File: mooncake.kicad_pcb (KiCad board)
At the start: 2 copper layers, 46 x 48.4 mm, 25 parts, among them U1 MCP23017, X1 Badgelife_shitty_connector

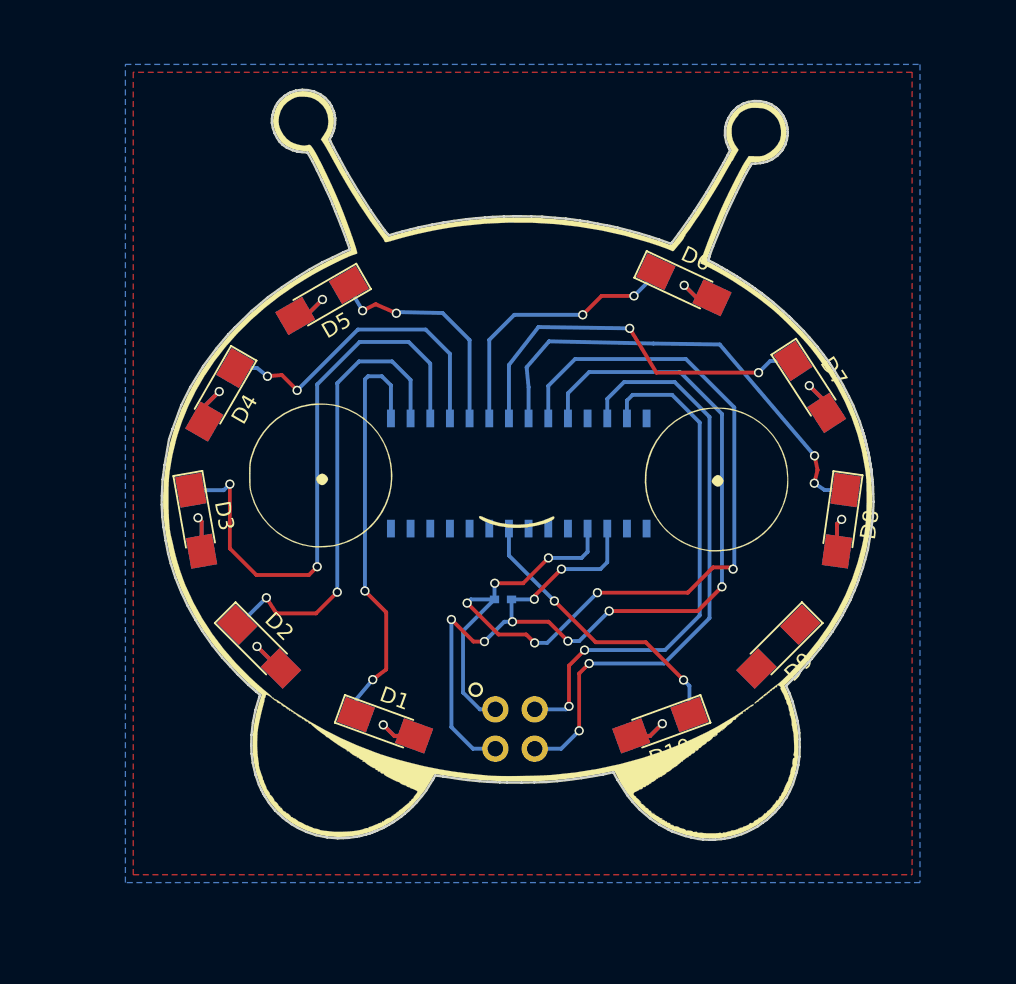
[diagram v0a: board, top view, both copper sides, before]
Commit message: Issues with EdgeCuts
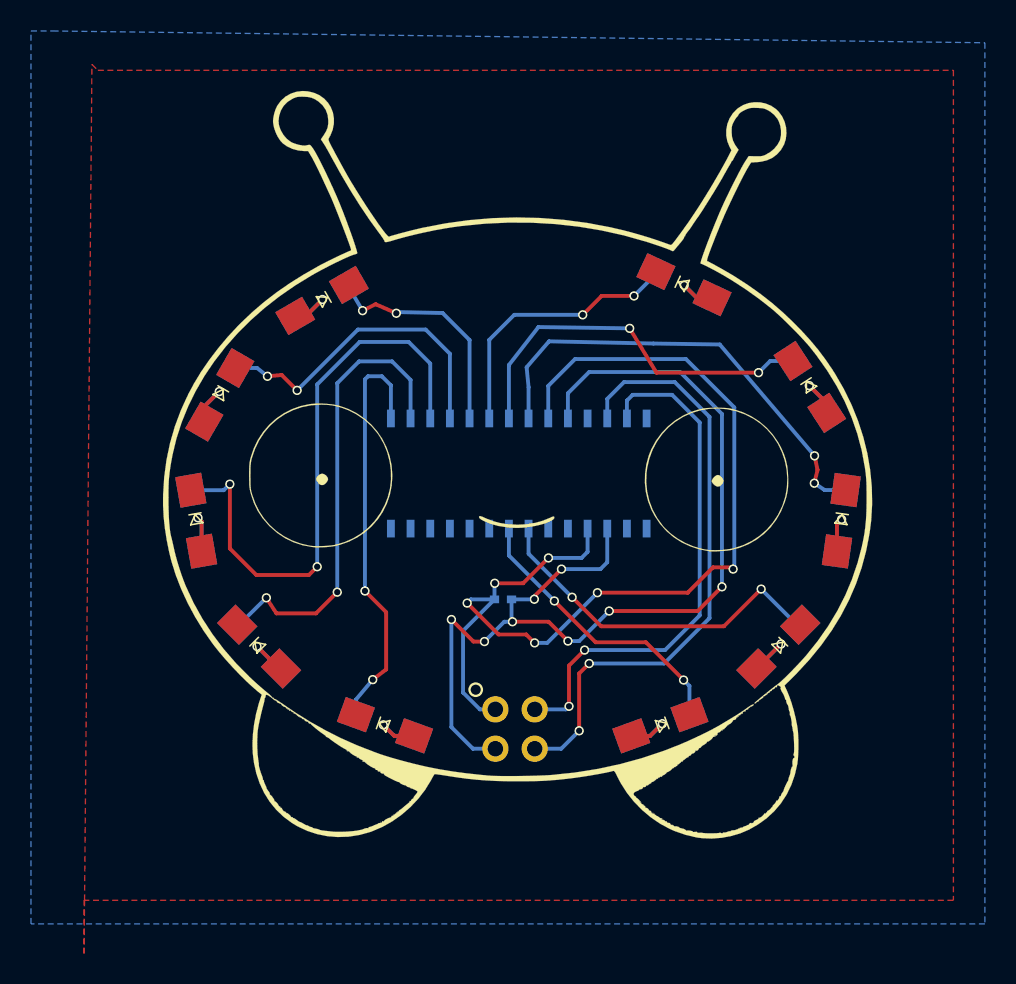
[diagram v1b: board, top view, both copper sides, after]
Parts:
- D1, D10, D2, D3, D4, D5, D6, D7, D8, D9: footprint LEDs:LED_1206_HandSoldering -> mrmeeseeks-addon-lib:LED_1206_HandSoldering_MinSilk
- R1, R10, R2, R3, R4, R5, R6, R7, R8, R9: footprint Resistors_SMD:R_1206_HandSoldering -> mrmeeseeks-addon-lib:R_1206_HandSoldering_NoSilk
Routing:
- net Net-(R9-Pad1): track 0.00 -> 23.1 mm, vias 0 -> 2
- net Net-(D9-Pad2): track 0.00 -> 4.48 mm, vias 0 -> 1
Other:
- board outline removed
- board text added: "#badgelife"
- board text added: "Thank you: AND!XOR SparX"

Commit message: Updated Traces
Gerbers included
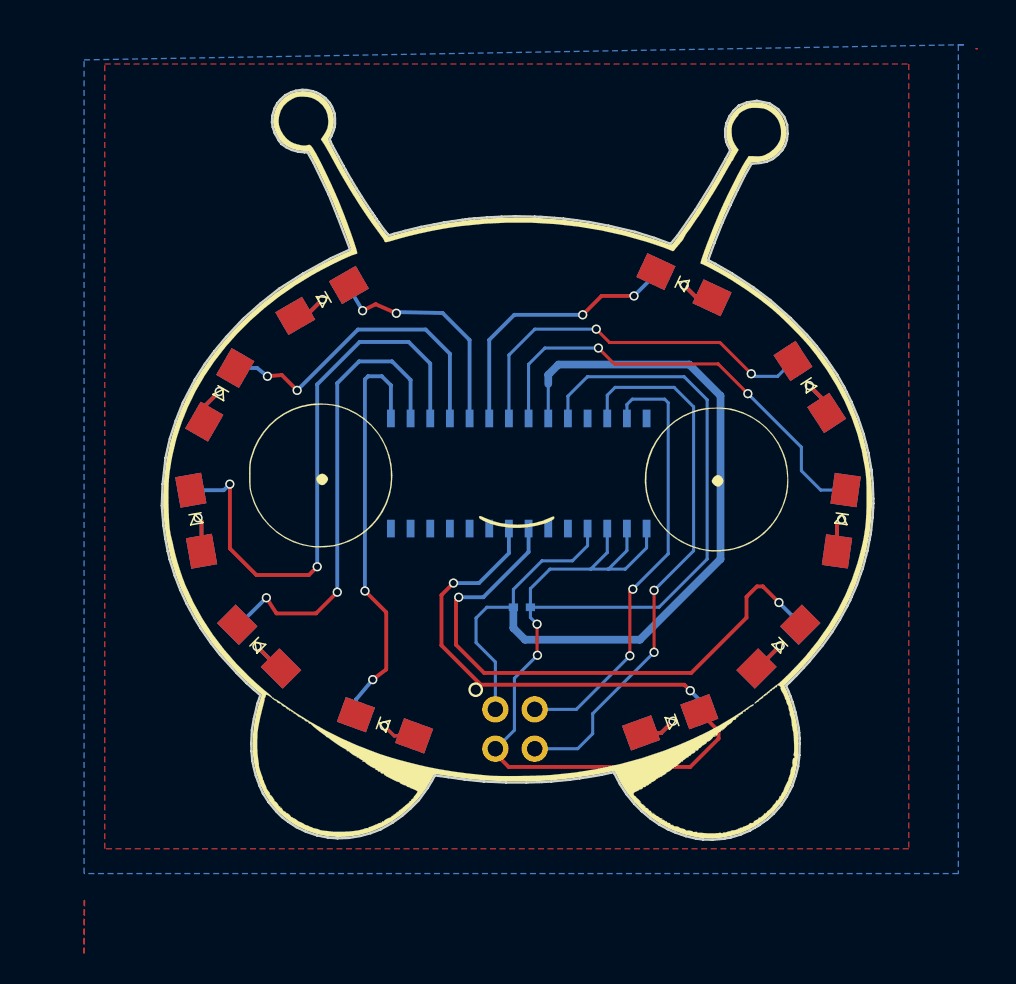
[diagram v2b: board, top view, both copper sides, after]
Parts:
- C1: footprint Capacitors_SMD:C_0402_NoSilk -> mrmeeseeks-addon-lib:C_0402_NoSilk_NoText
- moved C1 1.32 mm to (100.3, 109.2)
- moved D10 0.66 mm to (109.9, 116.6)
- moved R10 0.66 mm to (109.9, 116.6)
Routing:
- net Net-(R9-Pad1): track 23.1 -> 37.5 mm
- net GND: track 66.3 -> 80.3 mm, vias 8 -> 2
- net Net-(R10-Pad1): track 18.7 -> 29.3 mm
- net +3V3: track 67.6 -> 60.1 mm, vias 6 -> 0
- net sda: track 33.9 -> 28.8 mm
- net scl: track 39.2 -> 35.8 mm
- net Net-(R8-Pad1): track 30.0 -> 29.1 mm
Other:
- board outline added: 45.9 x 48.4 mm
